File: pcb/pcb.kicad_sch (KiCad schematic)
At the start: 37 parts, among them J1 USB_C_Receptacle_USB2.0_14P, J2 Conn_01x20, J3 Conn_01x20, J4 Conn_01x03, SW1 SW_Push, U1 RP2040, U2 NCP1117-3.3_SOT223, U3 W25Q128JVS, Y1 12 MHz

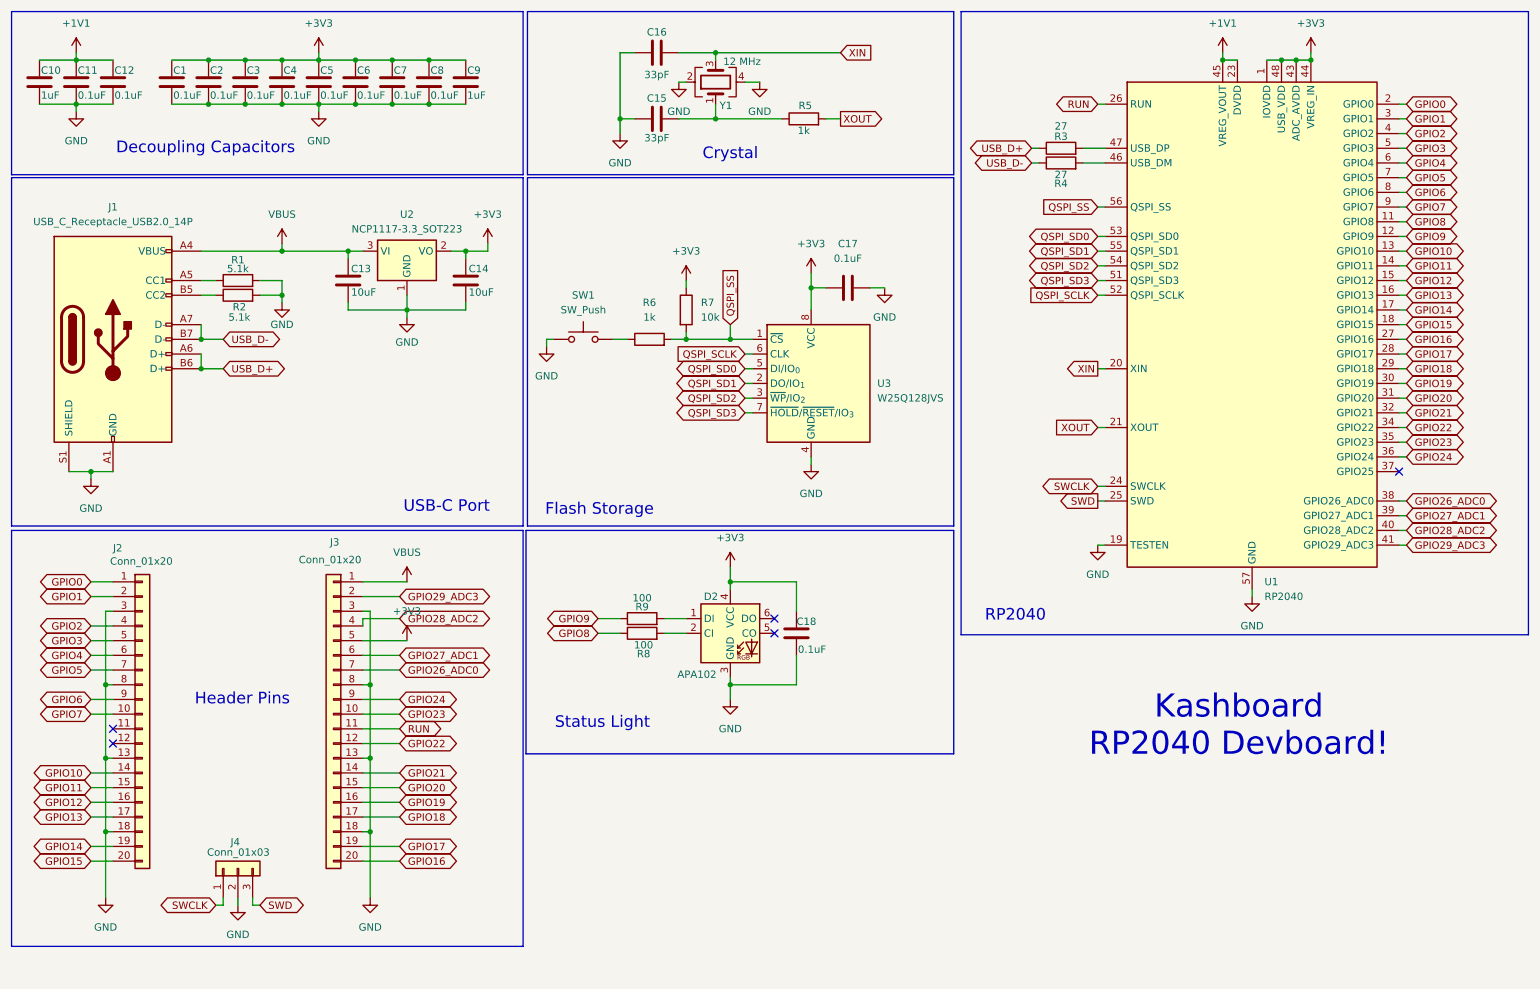
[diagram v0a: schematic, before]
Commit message: feat: updated most of the pcb, still have some capacitors to wire
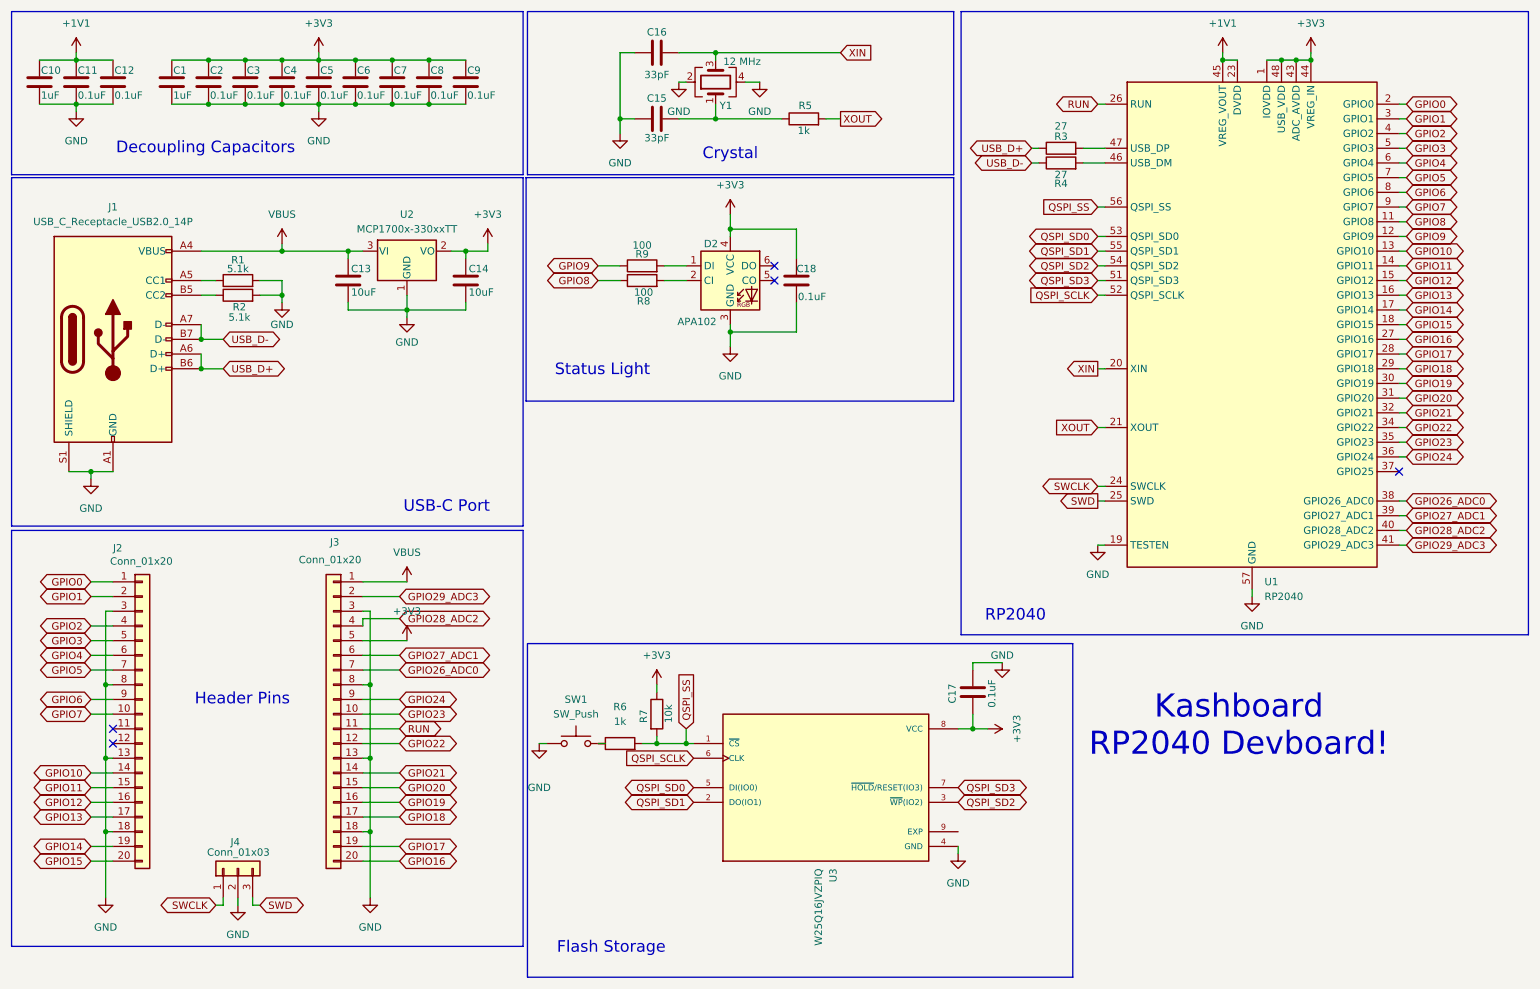
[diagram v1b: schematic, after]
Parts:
- removed U2: NCP1117-3.3_SOT223, Package_TO_SOT_SMD:SOT-223-3_TabPin2, symbol Regulator_Linear:NCP1117-3.3_SOT223
- removed U3: W25Q128JVS, Package_SO:SOIC-8_5.3x5.3mm_P1.27mm, symbol Memory_Flash:W25Q128JVS
- added U2: MCP1700x-330xxTT, Package_TO_SOT_SMD:SOT-23, symbol Regulator_Linear:MCP1700x-330xxTT
- added U3: W25Q16JVZPIQ, Package_SON:Winbond_USON-8-1EP_3x2mm_P0.5mm_EP0.2x1.6mm, symbol W25Q16JVZPIQ:W25Q16JVZPIQ
- C1: value 0.1uF -> 1uF
- C18: footprint (none) -> Capacitor_SMD:C_0402_1005Metric
- C9: value 1uF -> 0.1uF
- R8, R9: footprint (none) -> Resistor_SMD:R_0402_1005Metric
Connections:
- net +3V3: now also C17.2, U2.2 (VO), U3.8 (VCC); no longer C17.1
- net GND: now also C17.1, U2.1 (GND), U3.4 (GND); no longer C17.2
- net QSPI_SCLK: now also U3.6 (CLK)
- net QSPI_SD0: now also U3.5 (DI(IO0))
- net QSPI_SD1: now also U3.2 (DO(IO1))
- net QSPI_SD2: now also U3.3 (~{WP}(IO2))
- net QSPI_SD3: now also U3.7 (~{HOLD}/RESET(IO3))
- net QSPI_SS: now also U3.1 (~{CS})
- net VBUS: now also U2.3 (VI)
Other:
- moved on the sheet: C17, C18, D2, R6, R7, R8, R9, SW1

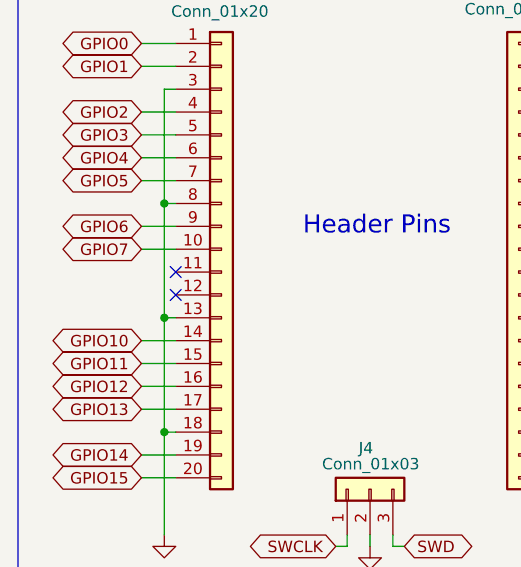
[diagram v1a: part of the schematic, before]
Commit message: holy shit massive update the pcb routing is done
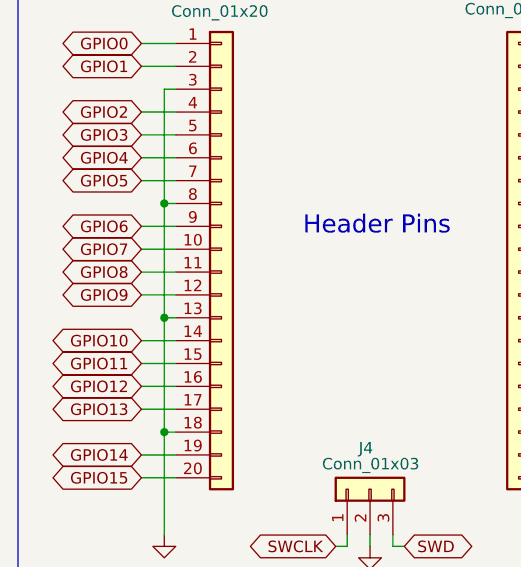
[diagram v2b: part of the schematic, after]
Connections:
- net GPIO8: now also J2.11 (Pin_11)
- net GPIO9: now also J2.12 (Pin_12)
- no-connect marks 5 -> 3
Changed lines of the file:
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@@
 		(at 254 93.98)
 	)
-	(no_connect
-		(at 31.75 140.97)
-	)
-	(no_connect
-		(at 31.75 138.43)
+	(wire
+		(pts
+			(xy 27.94 140.97) (xy 31.75 140.97)
+		)
+		(stroke
+			(width 0)
+			(type default)
+		)
 	)
 	(wire
@@
 		(pts
 			(xy 74.93 125.73) (xy 81.28 125.73)
+		)
+		(stroke
+			(width 0)
+			(type default)
+		)
+	)
+	(wire
+		(pts
+			(xy 27.94 138.43) (xy 31.75 138.43)
 		)
 		(stroke
@@
 		)
 	)
+	(global_label "GPIO8"
+		(shape bidirectional)
+		(at 27.94 138.43 180)
+		(fields_autoplaced yes)
+		(effects
+			(font
+				(size 1.27 1.27)
+			)
+			(justify right)
+		)
+		(property "Intersheetrefs" "${INTERSHEET_REFS}"
+			(at 18.1587 138.43 0)
+			(effects
+				(font
+					(size 1.27 1.27)
+				)
+				(justify right)
+				(hide yes)
+			)
+		)
+	)
 	(global_label "GPIO22"
 		(shape bidirectional)
@@
 				(hide yes)
 			)
+		)
+	)
+	(global_label "GPIO9"
+		(shape bidirectional)
+		(at 27.94 140.97 180)
+		(fields_autoplaced yes)
+		(effects
+			(font
+				(size 1.27 1.27)
+			)
+			(justify right)
+		)
+		(property "Intersheetrefs" "${INTERSHEET_REFS}"
+			(at 18.1587 140.97 0)
+			(effects
+				(font
+					(size 1.27 1.27)
+				)
+				(justify right)
+				(hide yes)
+			)
